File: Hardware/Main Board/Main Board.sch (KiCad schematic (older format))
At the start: 8 parts, among them Q1 NPN

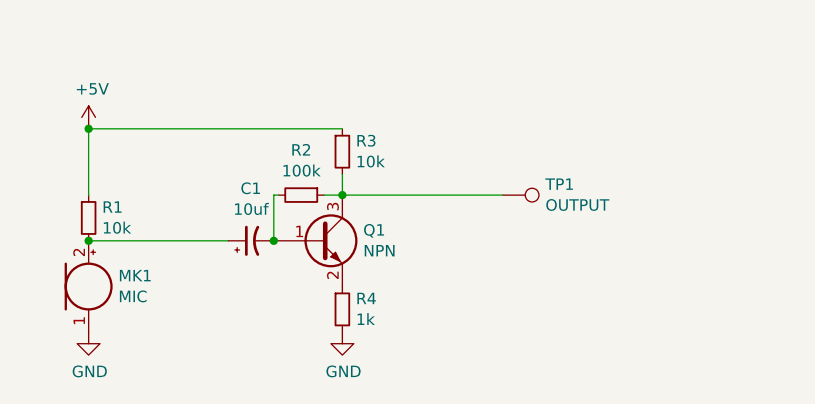
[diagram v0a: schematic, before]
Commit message: schemaic
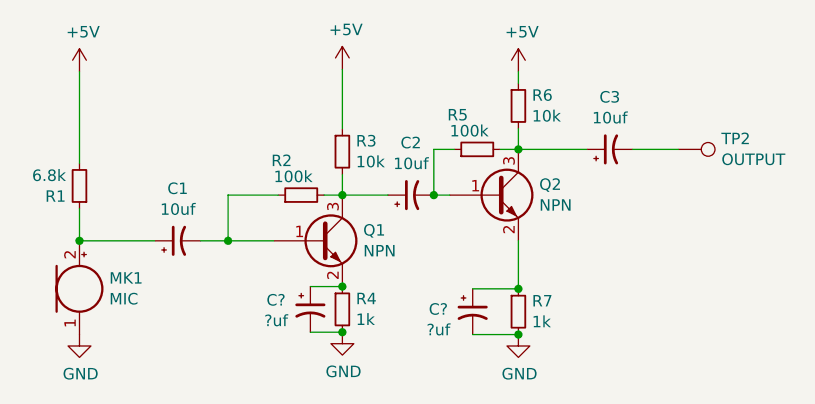
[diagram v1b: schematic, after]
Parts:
- removed TP1: OUTPUT, symbol Connector:TestPoint
- added C2, C3: 10uf, symbol Device:CP1_Small
- added C? (x2): ?uf, symbol Device:CP1_Small
- added Q2: NPN, symbol Device:Q_NPN_BEC
- added R5: 100k, symbol Device:R_Small
- added R6: 10k, symbol Device:R_Small
- added R7: 1k, symbol Device:R_Small
- added TP2: OUTPUT, symbol Connector:TestPoint
- R1: value 10k -> 6.8k
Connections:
- net +5V: now also R1.2, R6.1; no longer R1.1
- net GND: now also C?.2, C?.2, R7.2
- net at C1.1, MK1.2 (+): now also R1.1; no longer R1.2
- net at C1.2, Q1.1 (B): now also R2.1; no longer R2.2
- net at Q1.2 (E), R4.1: now also C?.1
- net at Q1.3 (C), R3.2: now also R2.2, C2.1; no longer R2.1
- new net: C2.2, Q2.1 (B), R5.1
- new net: C3.1, Q2.3 (C), R5.2, R6.2
- new net: C3.2, TP2.1
- new net: C?.1, Q2.2 (E), R7.1
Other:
- moved on the sheet: C1, MK1
